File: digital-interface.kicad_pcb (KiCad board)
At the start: 2 copper layers, 33 parts, among them U701 Si8641BD-B-IS2, U702 R05C05TE05S

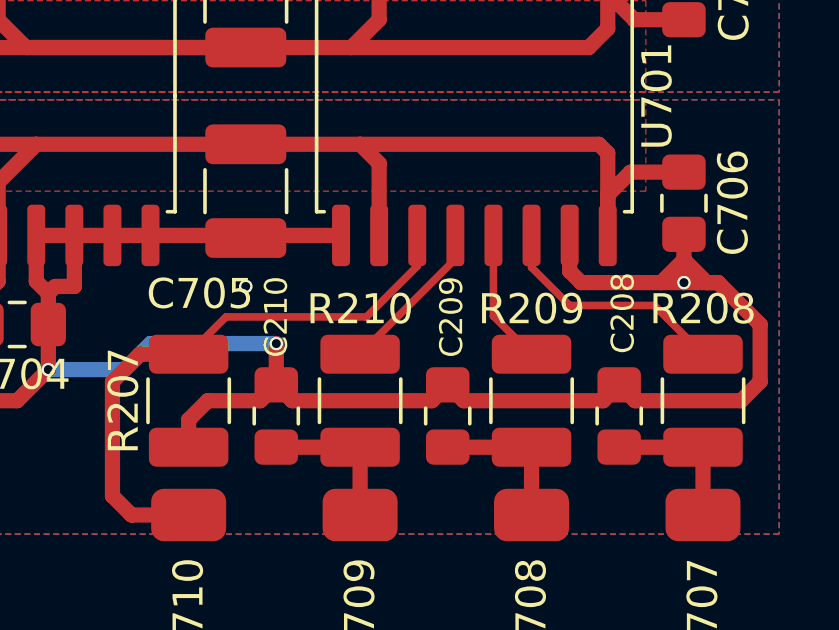
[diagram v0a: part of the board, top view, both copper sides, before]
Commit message: fix drc errors
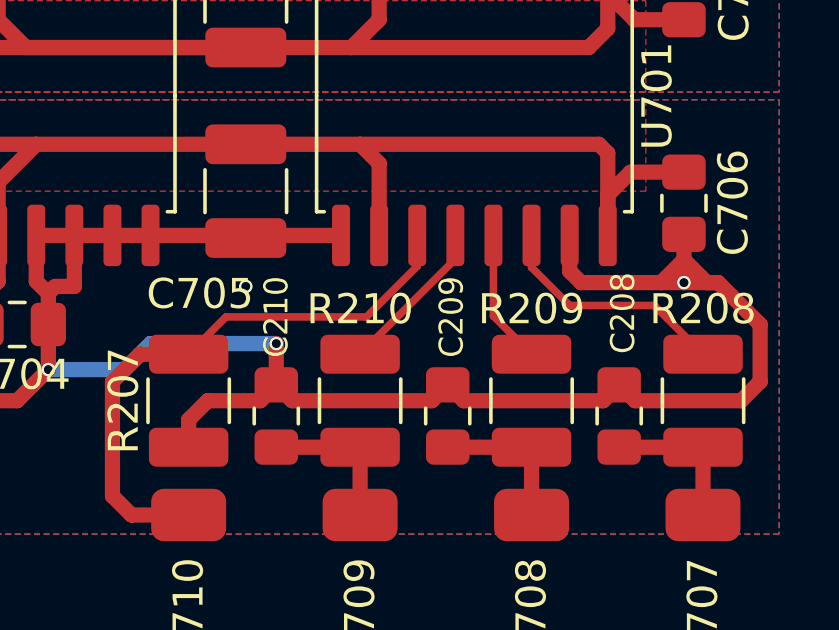
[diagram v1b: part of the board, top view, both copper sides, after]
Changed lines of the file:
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@@
 			(effects
 				(font
-					(size 0.762 0.762)
+					(size 0.8001 0.762)
 					(thickness 0.15)
 				)
@@
 			(effects
 				(font
-					(size 0.762 0.762)
+					(size 0.8001 0.762)
 					(thickness 0.15)
 				)
@@
 			(effects
 				(font
-					(size 0.762 0.762)
+					(size 0.8001 0.762)
 					(thickness 0.15)
 				)
